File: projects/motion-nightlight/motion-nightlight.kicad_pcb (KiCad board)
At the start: 2 copper layers, 48 x 50 mm, 19 parts, among them Q1 DARK_NPN_EBC, Q2 LED_CONTROL_NPN, SW1 SW_Push, SW2 SENSOR, SW3 MODE, U1 74HC14, U2 74LS08

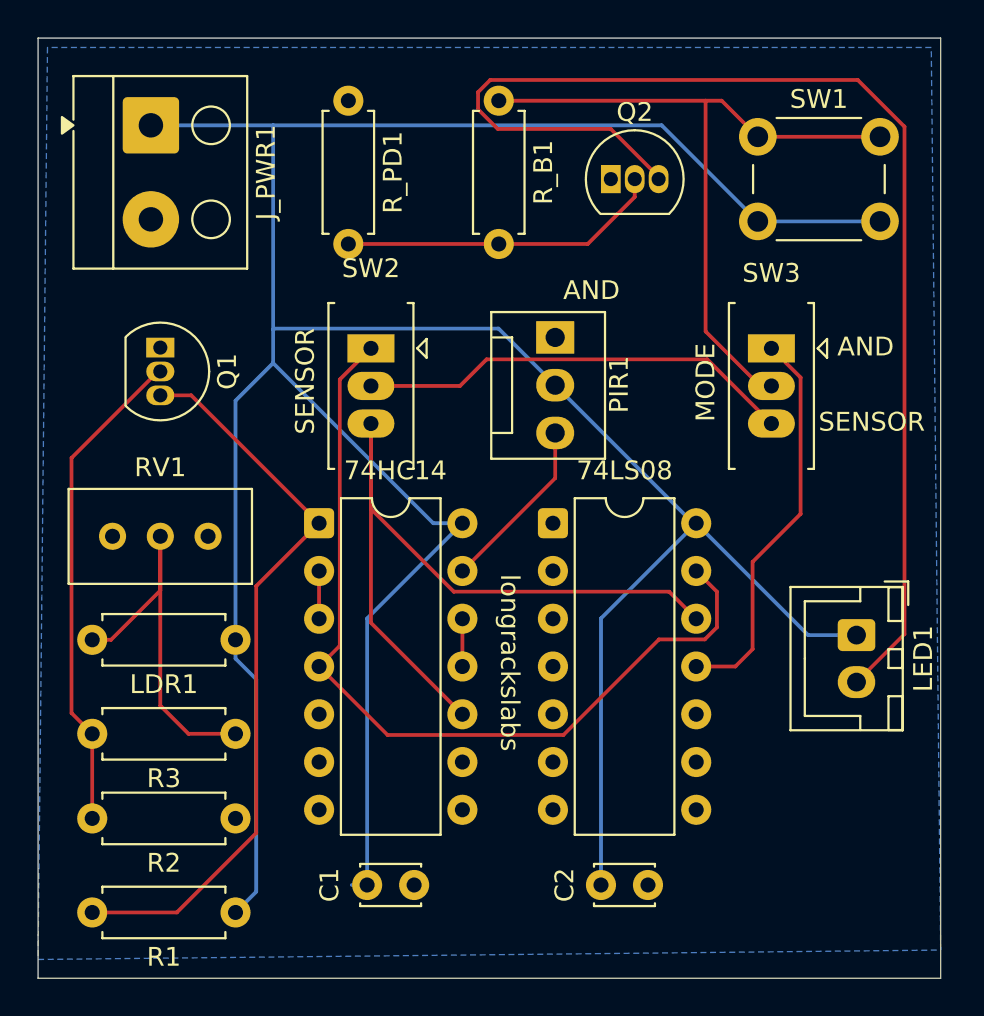
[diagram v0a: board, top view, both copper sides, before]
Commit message: clean ERC and DRC
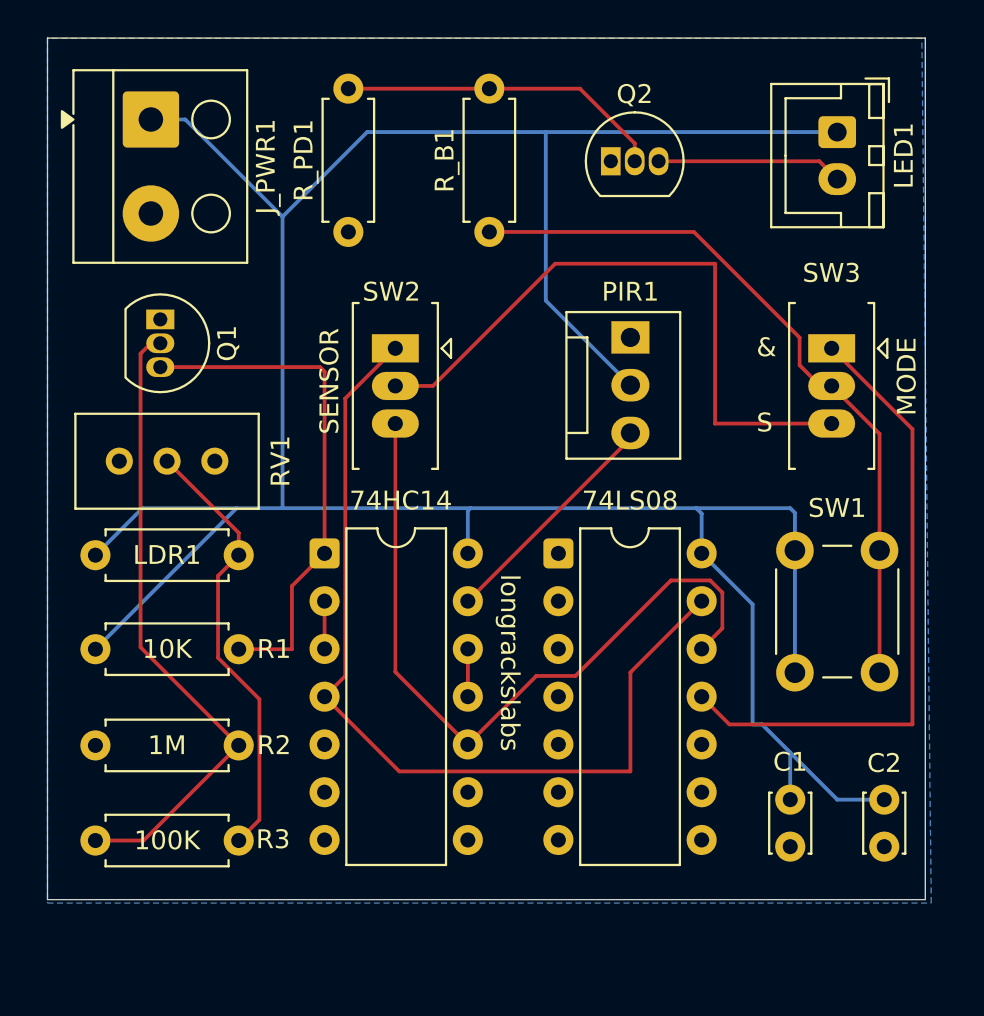
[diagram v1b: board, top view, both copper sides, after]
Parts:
- moved LED1 26.8 mm to (156.5, 72.0)
- moved C1 23.0 mm to (154.0, 107.5), turned to -90 degrees
- moved SW1 22.9 mm to (158.8, 94.2), turned to -90 degrees
- moved R1 15.9 mm to (117.0, 99.5), turned to 0 degrees
- moved C2 15.7 mm to (159.0, 107.5), turned to -90 degrees
- moved LDR1 8.70 mm to (117.0, 94.5), turned to 0 degrees
- moved R2 8.40 mm to (117.0, 104.6), turned to 0 degrees
- moved R_B1 7.00 mm to (138.0, 77.3), turned to 90 degrees
- moved R_PD1 6.98 mm to (130.5, 77.3), turned to 90 degrees
- moved R3 5.68 mm to (124.7, 109.7)
- moved RV1 4.01 mm to (123.4, 89.5)
- moved PIR1 4.00 mm to (145.5, 82.9)
- moved SW3 3.20 mm to (156.2, 83.5)
- moved U1 1.63 mm to (129.2, 94.4)
- moved U2 1.63 mm to (141.7, 94.4)
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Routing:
- net /LED_ON: track 66.7 -> 9.89 mm
- net +3.3V: track 179.4 -> 156.1 mm
- net /AND_ON: track 21.1 -> 33.6 mm
- net /DARK_RAW: track 39.6 -> 27.3 mm
- net /SENSOR_DIG: track 23.3 -> 34.4 mm
- net Net-(Q1-B): track 26.3 -> 34.0 mm
- net /MOTION_RAW: track 9.38 -> 12.8 mm
- net Net-(LDR1-Pad2): track 21.2 -> 23.6 mm
- net /MOTION_DIG: track 41.7 -> 39.5 mm
- net /DARK_DIG: track 46.5 -> 48.6 mm
- net /LIGHT_ON: track 38.1 -> 38.8 mm
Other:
- board size 48 x 50 mm -> 46.7 x 45.8 mm
- board text added: "&"
- board text added: "S"
- board text removed: "AND"
- board text removed: "SENSOR"
